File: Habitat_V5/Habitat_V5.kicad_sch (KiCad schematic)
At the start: 102 parts, among them J2 Conn_01x03_Socket, J3 Conn_01x12, J4 Conn_01x03_Socket, J5 Conn_01x03_Socket, K1 Relay_SPDT, Q1 PMOS, Q2 2N7002K, Q3 40N02, U1 XL1509-5V, U2 AP2112K-3.3, U3 PC817, U6 ESP32-WROOM-32

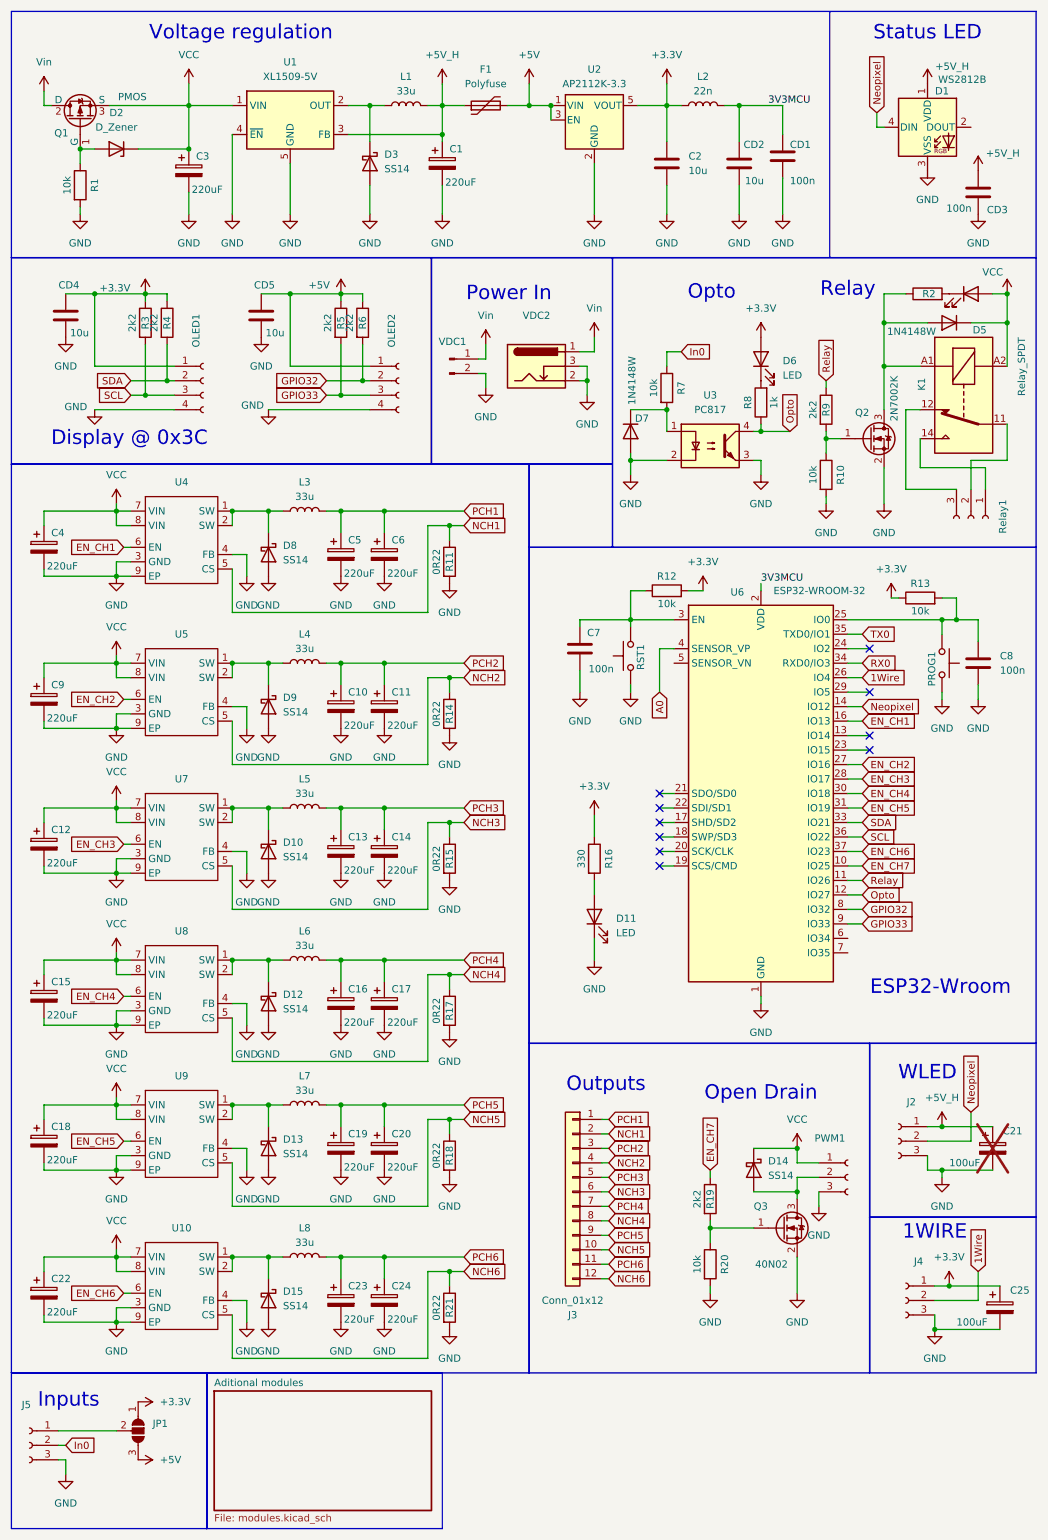
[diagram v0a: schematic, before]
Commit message: Updated PCB and Schematic
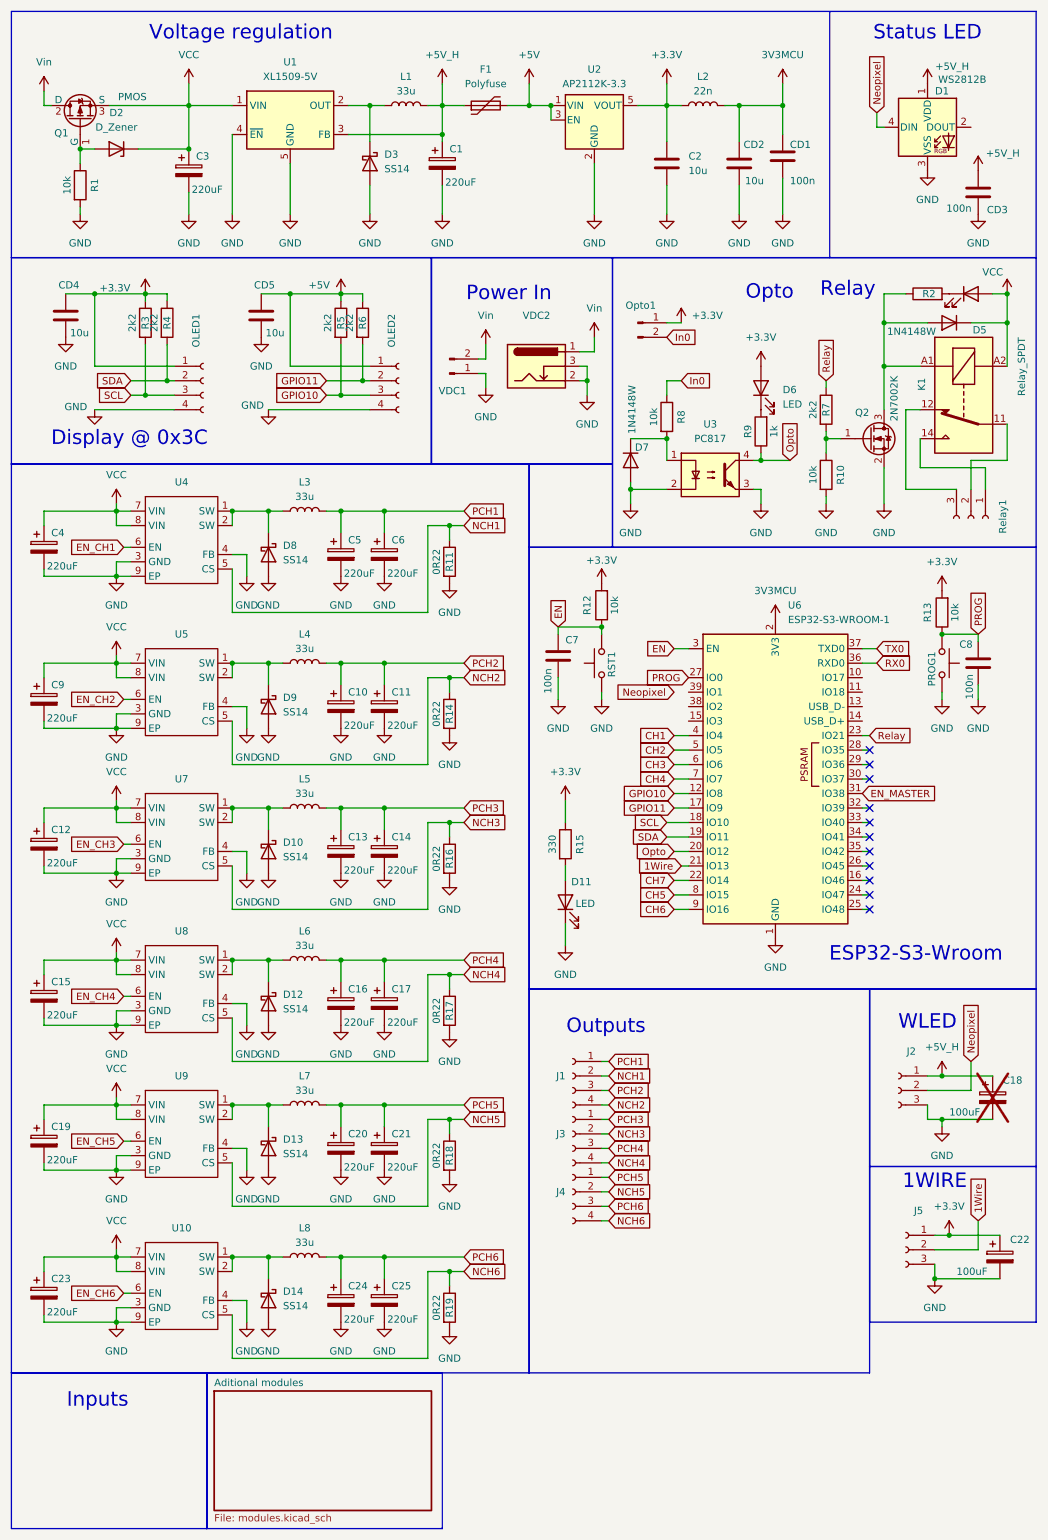
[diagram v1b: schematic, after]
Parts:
- removed D14: SS14, Diode_SMD:D_SMA, symbol Diode:SS14
- removed J3: Conn_01x12, Connector_Phoenix_GMSTB:PhoenixContact_GMSTBVA_2,5_12-G-7,62_1x12_P7.62mm_Vertical, symbol Connector_Generic:Conn_01x12
- removed J5, PWM1: Conn_01x03_Socket, TerminalBlock_Phoenix:TerminalBlock_Phoenix_MKDS-1,5-3_1x03_P5.00mm_Horizontal, symbol Connector:Conn_01x03_Socket
- removed JP1: SolderJumper_3_Open, Jumper:SolderJumper-3_P2.0mm_Open_TrianglePad1.0x1.5mm, symbol Jumper:SolderJumper_3_Open
- removed Q3: 40N02, Package_TO_SOT_SMD:TO-252-2, symbol Transistor_FET:2N7002K
- removed R19: 2k2, Resistor_SMD:R_0805_2012Metric, symbol Device:R
- removed R20: 10k, Resistor_SMD:R_0805_2012Metric, symbol Device:R
- removed U6: ESP32-WROOM-32, RF_Module:ESP32-WROOM-32, symbol RF_Module:ESP32-WROOM-32
- added J1, J3, J4: Conn_01x04_Socket, Connector_Phoenix_MSTB:PhoenixContact_MSTBA_2,5_4-G-5,08_1x04_P5.08mm_Horizontal, symbol Connector:Conn_01x04_Socket
- added Opto1: Conn_01x02_Pin, Connector_Phoenix_MSTB:PhoenixContact_MSTBA_2,5_2-G-5,08_1x02_P5.08mm_Horizontal, symbol Connector:Conn_01x02_Pin
- added U6: ESP32-S3-WROOM-1, RF_Module:ESP32-S3-WROOM-1, symbol RF_Module:ESP32-S3-WROOM-1
- J2, Relay1: footprint TerminalBlock_Phoenix:TerminalBlock_Phoenix_MKDS-1,5-3_1x03_P5.00mm_Horizontal -> Connector_Phoenix_MSTB:PhoenixContact_MSTBA_2,5_3-G-5,08_1x03_P5.08mm_Horizontal
- J5: renamed from J4; footprint TerminalBlock_Phoenix:TerminalBlock_Phoenix_MKDS-1,5-3_1x03_P5.00mm_Horizontal -> Connector_Phoenix_MSTB:PhoenixContact_MSTBA_2,5_3-G-5,08_1x03_P5.08mm_Horizontal
- VDC1: footprint Connector_Phoenix_GMSTB:PhoenixContact_GMSTBVA_2,5_2-G-7,62_1x02_P7.62mm_Vertical -> Connector_Phoenix_MSTB:PhoenixContact_MSTBA_2,5_2-G-5,08_1x02_P5.08mm_Horizontal
- renumbered C21 to C18, C18 to C19, C19 to C20, C20 to C21, C25 to C22, C22 to C23, C23 to C24, C24 to C25, D15 to D14, R16 to R15, R15 to R16, R21 to R19, R9 to R7, R7 to R8, R8 to R9
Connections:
- net +3.3V: now also R13.2, Opto1.1 (Pin_1); no longer R13.1
- net 1Wire: now also U6.21 (IO13)
- net 3V3MCU: now also U6.2 (3V3)
- net GND: now also VDC1.1 (Pin_1), U6.1 (GND), U6.40 (GND), U6.41 (GND); no longer VDC1.2 (Pin_2)
- net In0: now also Opto1.2 (Pin_2)
- net NCH1: now also J1.2 (Pin_2)
- net NCH2: now also J1.4 (Pin_4)
- net NCH3: now also J3.2 (Pin_2)
- net NCH4: now also J3.4 (Pin_4)
- net NCH5: now also J4.2 (Pin_2)
- net NCH6: now also J4.4 (Pin_4)
- net Opto: now also U6.20 (IO12)
- net PCH1: now also J1.1 (Pin_1)
- net PCH2: now also J1.3 (Pin_3)
- net PCH3: now also J3.1 (Pin_1)
- net PCH4: now also J3.3 (Pin_3)
- net PCH5: now also J4.1 (Pin_1)
- net PCH6: now also J4.3 (Pin_3)
- net RX0: now also U6.36 (RXD0)
- net Relay: now also U6.23 (IO21)
- net SCL: now also U6.18 (IO10)
- net SDA: now also U6.19 (IO11)
- net TX0: now also U6.37 (TXD0)
- net Vin: now also VDC1.2 (Pin_2); no longer VDC1.1 (Pin_1)
- net EN: now reaches C7.1, R12.1, RST1.2
- net EN: now also U6.3 (EN)
- net PROG: now reaches C8.1, PROG1.2
- net PROG: now also R13.1, U6.27 (IO0); no longer R13.2
- net GPIO32 renamed GPIO11
- net GPIO11: now also U6.17 (IO9)
- net GPIO33 renamed GPIO10
- net GPIO10: now also U6.12 (IO8)
- new net CH1: U6.4 (IO4)
- new net CH2: U6.5 (IO5)
- new net CH3: U6.6 (IO6)
- new net CH4: U6.7 (IO7)
- new net CH5: U6.8 (IO15)
- new net CH6: U6.9 (IO16)
- new net CH7: U6.22 (IO14)
- new net EN_MASTER: U6.31 (IO38)
- no-connect marks 10 -> 11
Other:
- note added: "ESP32-S3-Wroom"
- note removed: "ESP32-Wroom"
- note removed: "Open Drain"
- moved on the sheet: C18, C22, C7, D11, D6, D7, J2, J5, R12, R13, R15, R8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
